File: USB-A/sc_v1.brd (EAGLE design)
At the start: 29.2 x 15.2 mm, 21 parts, among them IC1 CP2102, J2 USB_A_SMT_MALE, U2 3.3V

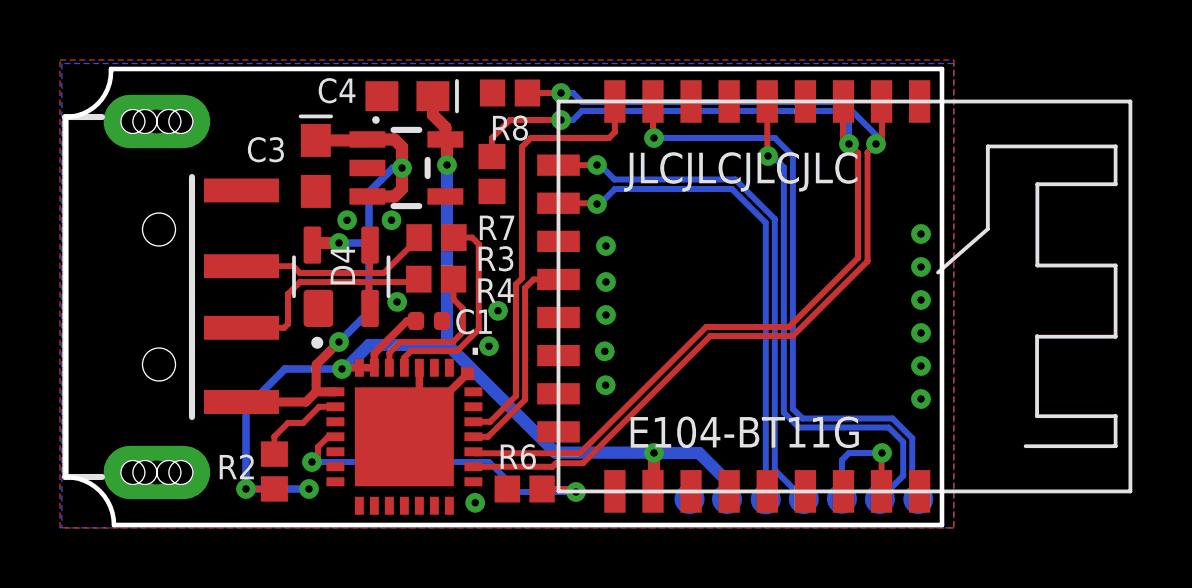
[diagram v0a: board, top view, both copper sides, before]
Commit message: Add files via upload
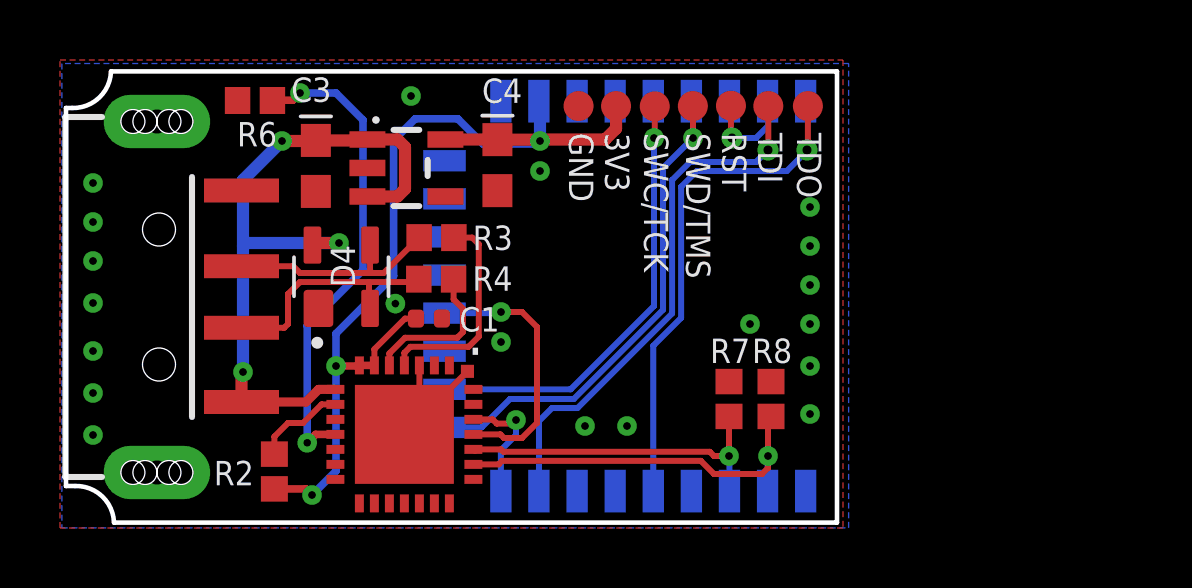
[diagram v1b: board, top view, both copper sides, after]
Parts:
- moved R6 15.8 mm to (21.7, 16.4)
- moved TP7 14.0 mm to (38.8, 16.3), flipped to the top
- moved TP1 13.6 mm to (32.5, 16.3), flipped to the top
- moved TP2 13.6 mm to (33.7, 16.3), flipped to the top
- moved TP3 13.6 mm to (35.0, 16.3), flipped to the top
- moved TP4 13.6 mm to (36.3, 16.3), flipped to the top
- moved TP5 13.6 mm to (37.6, 16.3), flipped to the top
- moved U$1 13.4 mm to (28.0, 3.47), flipped to the bottom, turned to 90 degrees
- moved R8 13.4 mm to (38.9, 6.50), turned to 90 degrees
- moved TP6 13.3 mm to (40.1, 16.3), flipped to the top
- moved R7 10.9 mm to (37.5, 6.50), turned to 90 degrees
- moved C4 3.78 mm to (29.8, 14.3), turned to 90 degrees
- moved C1 0.08 mm to (27.5, 9.18)
- moved IC1 0.08 mm to (26.7, 5.32)
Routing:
- net PB00: track 34.7 -> 11.2 mm, vias 2 -> 1
- net PB01: track 34.0 -> 13.1 mm, vias 2 -> 1
- net RX: track 14.5 -> 4.11 mm, vias 0 -> 1
- net +3V3: track 38.4 -> 31.5 mm, vias 5 -> 3
- net N$5: track 11.7 -> 16.1 mm
- net +5V: track 19.9 -> 23.9 mm
- net TDI: track 21.0 -> 17.8 mm
- net TCK: track 16.8 -> 14.8 mm
- net TX: track 7.19 -> 8.88 mm, vias 0 -> 1
- net TMS: track 17.7 -> 16.1 mm
- net RST: track 4.01 -> 3.29 mm
- net TDO: track 17.3 -> 16.7 mm
- net GND: track 4.76 -> 4.90 mm, vias 17 -> 20
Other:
- board size 29.2 x 15.2 mm -> 25.7 x 15 mm
